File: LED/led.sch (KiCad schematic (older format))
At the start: 4 parts

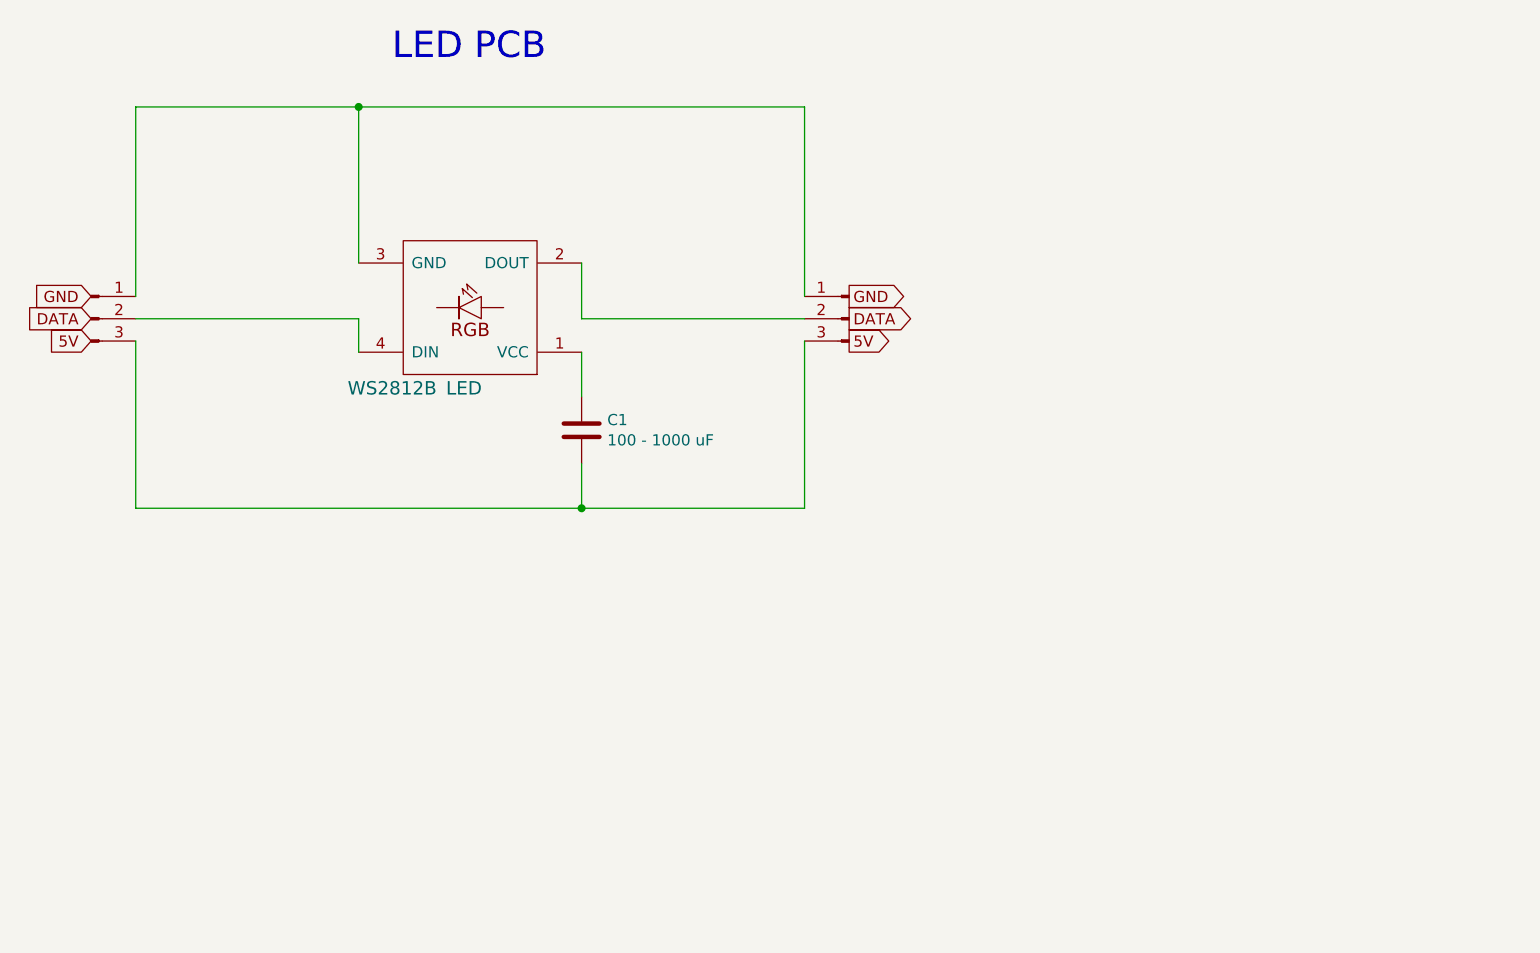
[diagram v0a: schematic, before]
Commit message: Finish LED scematics
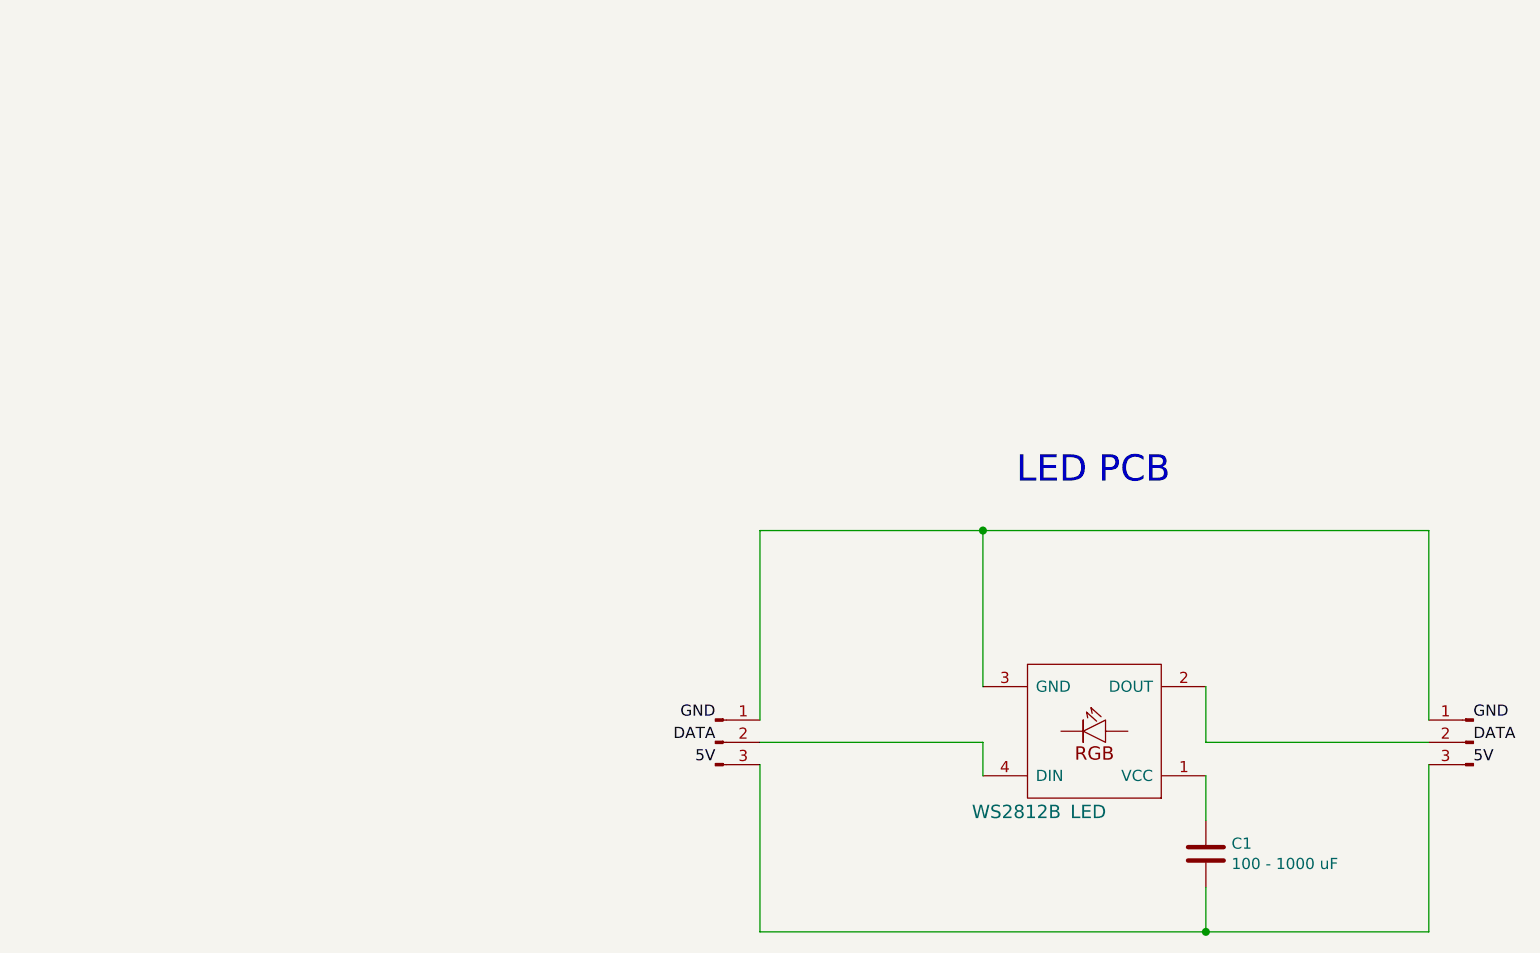
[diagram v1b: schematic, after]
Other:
- moved on the sheet: C1, LED
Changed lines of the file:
@@
 L Connector:Conn_01x03_Male J?
 U 1 1 607A4CB2
-P 1300 2050
-F 0 "J?" H 1408 2331 50  0001 C CNN
-F 1 "Conn_01x03_Male" H 1408 2240 50  0001 C CNN
-F 2 "" H 1300 2050 50  0001 C CNN
-F 3 "~" H 1300 2050 50  0001 C CNN
-	1    1300 2050
+P 4100 3950
+F 0 "J?" H 4208 4231 50  0001 C CNN
+F 1 "Conn_01x03_Male" H 4208 4140 50  0001 C CNN
+F 2 "" H 4100 3950 50  0001 C CNN
+F 3 "~" H 4100 3950 50  0001 C CNN
+	1    4100 3950
 	1    0    0    -1
 $EndComp
 Wire Wire Line
-	1500 2050 2500 2050
+	4300 3950 5300 3950
 Wire Wire Line
-	2500 2050 2500 2200
+	5300 3950 5300 4100
 $Comp
 L Connector:Conn_01x03_Male J?
 U 1 1 607A2A3A
-P 4700 2050
-F 0 "J?" H 4672 2074 50  0001 R CNN
-F 1 "Conn_01x03_Male" H 4672 1983 50  0001 R CNN
-F 2 "" H 4700 2050 50  0001 C CNN
-F 3 "~" H 4700 2050 50  0001 C CNN
-	1    4700 2050
+P 7500 3950
+F 0 "J?" H 7472 3974 50  0001 R CNN
+F 1 "Conn_01x03_Male" H 7472 3883 50  0001 R CNN
+F 2 "" H 7500 3950 50  0001 C CNN
+F 3 "~" H 7500 3950 50  0001 C CNN
+	1    7500 3950
 	-1   0    0    -1
 $EndComp
 Wire Wire Line
-	3500 2050 4500 2050
-Text GLabel 1300 1950 0    50   Input ~ 0
-GND
-Text GLabel 1300 2050 0    50   Input ~ 0
-DATA
-Text GLabel 4700 2050 2    50   Output ~ 0
-DATA
-Text GLabel 4700 2150 2    50   Output ~ 0
-5V
-Text GLabel 1300 2150 0    50   Input ~ 0
-5V
+	6300 3950 7300 3950
 Wire Wire Line
-	3500 1800 3500 2050
+	6300 3700 6300 3950
 $Comp
 L ws2812b:WS2812B LED
 U 1 1 6079C2AE
-P 3000 2000
-F 0 "LED" H 2947 2362 60  0000 L CNN
-F 1 "WS2812B" H 3150 2362 60  0000 L CNN
-F 2 "" V 2950 2000 60  0000 C CNN
-F 3 "" V 2950 2000 60  0000 C CNN
-	1    3000 2000
+P 5800 3900
+F 0 "LED" H 5747 4262 60  0000 L CNN
+F 1 "WS2812B" H 5950 4262 60  0000 L CNN
+F 2 "" V 5750 3900 60  0000 C CNN
+F 3 "" V 5750 3900 60  0000 C CNN
+	1    5800 3900
 	-1   0    0    1
 $EndComp
 Wire Wire Line
-	1500 1100 2500 1100
+	4300 3000 5300 3000
 Wire Wire Line
-	1500 2900 3500 2900
-Connection ~ 2500 1100
+	4300 4800 6300 4800
+Connection ~ 5300 3000
 Wire Wire Line
-	2500 1100 4500 1100
-Connection ~ 3500 2900
+	5300 3000 7300 3000
+Connection ~ 6300 4800
 Wire Wire Line
-	3500 2900 4500 2900
+	6300 4800 7300 4800
 Wire Wire Line
-	4500 2150 4500 2900
+	7300 4050 7300 4800
 Wire Wire Line
-	1500 2150 1500 2900
+	4300 4050 4300 4800
 Wire Wire Line
-	1500 1100 1500 1950
+	4300 3000 4300 3850
 Wire Wire Line
-	4500 1100 4500 1950
+	7300 3000 7300 3850
 Wire Wire Line
-	3500 2200 3500 2400
+	6300 4100 6300 4300
 Wire Wire Line
-	2500 1800 2500 1100
+	5300 3700 5300 3000
 $Comp
 L Device:C C1
 U 1 1 607F11E7
-P 3500 2550
-F 0 "C1" H 3615 2596 50  0000 L CNN
-F 1 "100 - 1000 uF" H 3615 2505 50  0000 L CNN
-F 2 "" H 3538 2400 50  0001 C CNN
-F 3 "~" H 3500 2550 50  0001 C CNN
-	1    3500 2550
+P 6300 4450
+F 0 "C1" H 6415 4496 50  0000 L CNN
+F 1 "100 - 1000 uF" H 6415 4405 50  0000 L CNN
+F 2 "" H 6338 4300 50  0001 C CNN
+F 3 "~" H 6300 4450 50  0001 C CNN
+	1    6300 4450
 	1    0    0    -1
 $EndComp
 Wire Wire Line
-	3500 2700 3500 2900
-Text Notes 2650 900  0    118  ~ 0
+	6300 4600 6300 4800
+Text Notes 5450 2800 0    118  ~ 0
 LED PCB
-Text GLabel 4700 1950 2    50   Output ~ 0
+Text Label 4100 3850 2    50   ~ 0
 GND
+Text Label 4100 3950 2    50   ~ 0
+DATA
+Text Label 4100 4050 2    50   ~ 0
+5V
+Text Label 7500 3850 0    50   ~ 0
+GND
+Text Label 7500 3950 0    50   ~ 0
+DATA
+Text Label 7500 4050 0    50   ~ 0
+5V
 $EndSCHEMATC
